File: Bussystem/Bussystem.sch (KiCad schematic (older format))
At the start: 11 parts, among them J1 PCIE-098-02-X-D-TH, J2 PCIE-098-02-X-D-TH, J3 PCIE-098-02-X-D-TH, J4 PCIE-098-02-X-D-TH, J5 PCIE-098-02-X-D-TH, J6 PCIE-098-02-X-D-EMS2-BG, J7 8x Edge conn

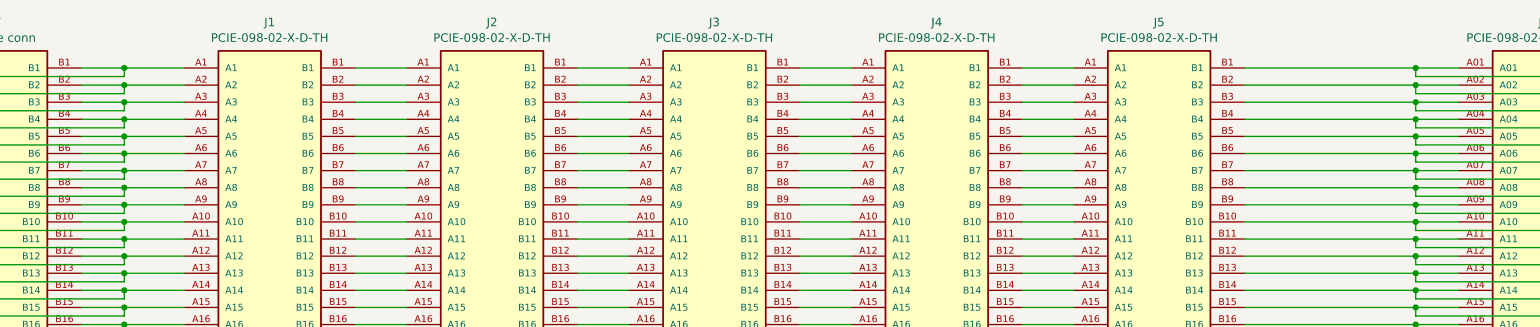
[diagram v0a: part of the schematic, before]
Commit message: lanes
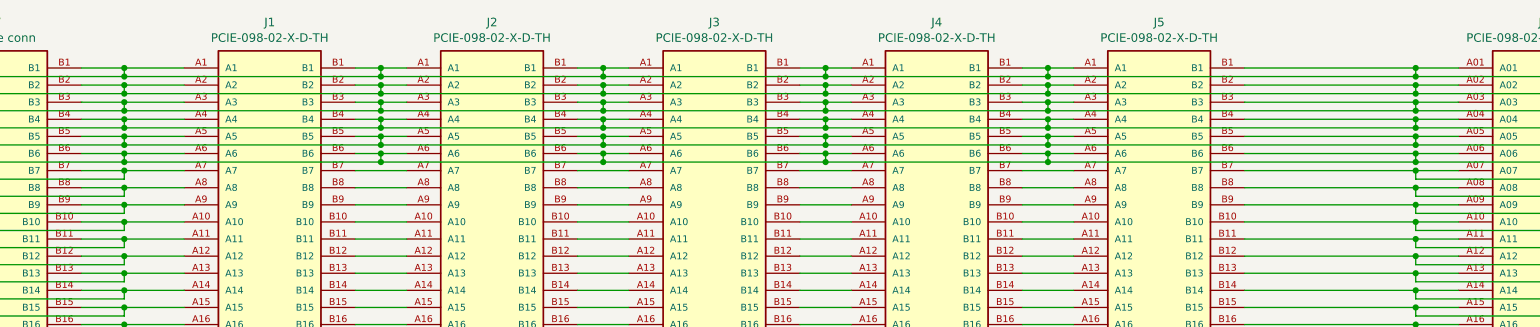
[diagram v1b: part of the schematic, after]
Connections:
- net at J1.A1, J7.A1, J7.B1: now also J1.B1, J2.A1, J2.B1, J3.A1, J3.B1, J4.A1, J4.B1, J5.A1, J5.B1, J6.A01, J6.B01
- net at J1.A2, J7.A2, J7.B2: now also J1.B2, J2.A2, J2.B2, J3.A2, J3.B2, J4.A2, J4.B2, J5.A2, J5.B2, J6.A02, J6.B02
- net at J1.A3, J7.A3, J7.B3: now also J1.B3, J2.A3, J2.B3, J3.A3, J3.B3, J4.A3, J4.B3, J5.A3, J5.B3, J6.A03, J6.B03
- net at J1.A4, J7.A4, J7.B4: now also J1.B4, J2.A4, J2.B4, J3.A4, J3.B4, J4.A4, J4.B4, J5.A4, J5.B4, J6.A04, J6.B04
- net at J1.A5, J7.A5, J7.B5: now also J1.B5, J2.A5, J2.B5, J3.A5, J3.B5, J4.A5, J4.B5, J5.A5, J5.B5, J6.A05, J6.B05
- net at J1.A6, J7.A6, J7.B6: now also J1.B6, J2.A6, J2.B6, J3.A6, J3.B6, J4.A6, J4.B6, J5.A6, J5.B6, J6.A06, J6.B06

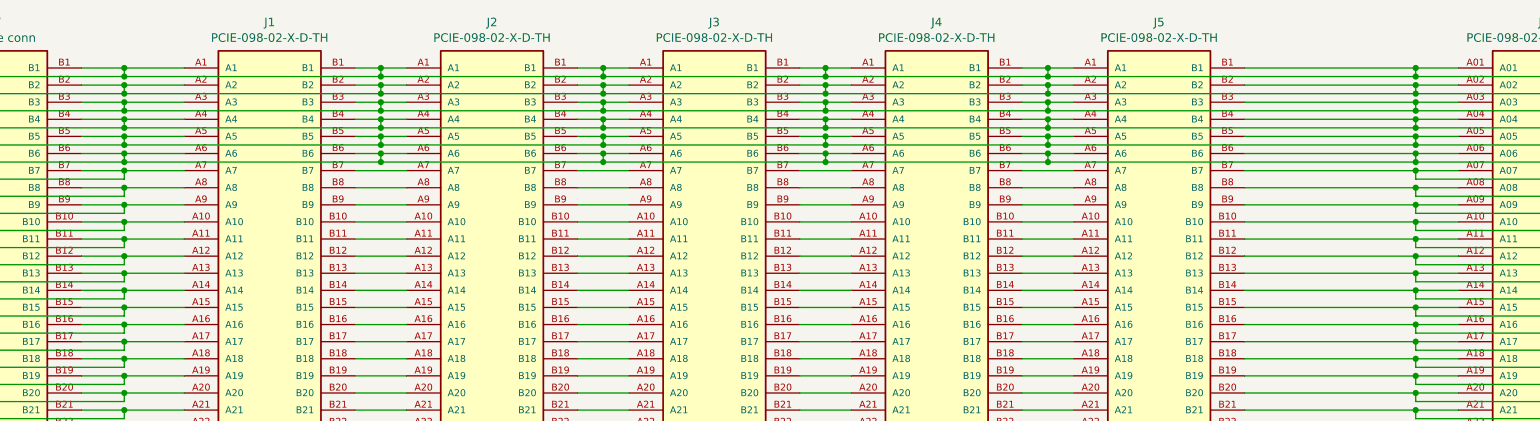
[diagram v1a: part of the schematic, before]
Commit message: some step files and additional editing of the sch
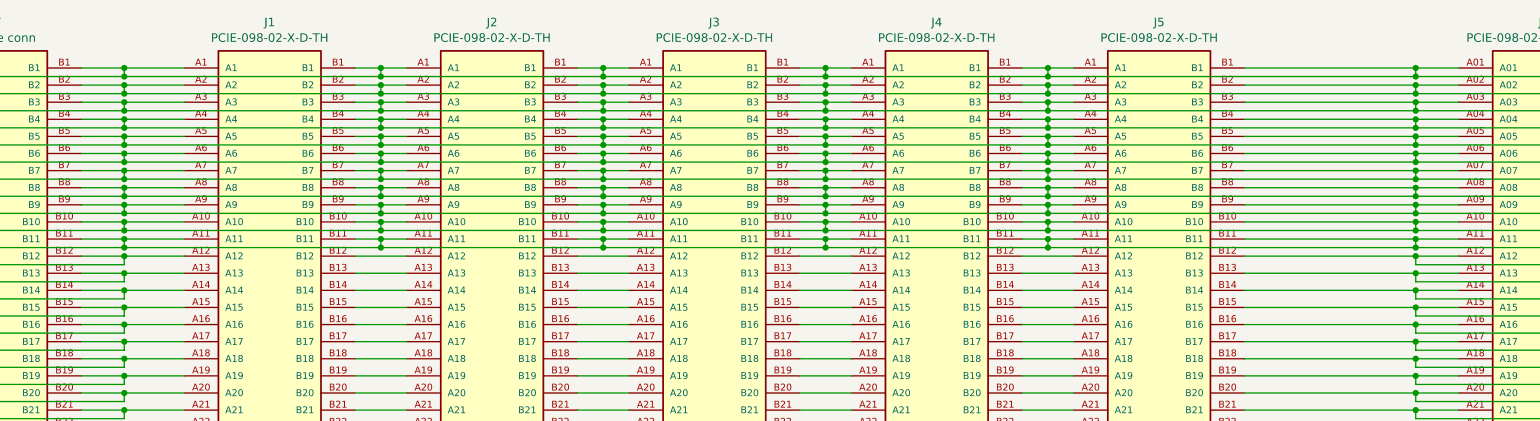
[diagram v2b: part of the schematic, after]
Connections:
- net at J1.A10, J7.A10, J7.B10: now also J1.B10, J2.A10, J2.B10, J3.A10, J3.B10, J4.A10, J4.B10, J5.A10, J5.B10, J6.A10, J6.B10
- net at J1.A11, J7.A11, J7.B11: now also J1.B11, J2.A11, J2.B11, J3.A11, J3.B11, J4.A11, J4.B11, J5.A11, J5.B11, J6.A11, J6.B11
- net at J1.A7, J7.A7, J7.B7: now also J1.B7, J2.A7, J2.B7, J3.A7, J3.B7, J4.A7, J4.B7, J5.A7, J5.B7, J6.A07, J6.B07
- net at J1.A8, J7.A8, J7.B8: now also J1.B8, J2.A8, J2.B8, J3.A8, J3.B8, J4.A8, J4.B8, J5.A8, J5.B8, J6.A08, J6.B08
- net at J1.A9, J7.A9, J7.B9: now also J1.B9, J2.A9, J2.B9, J3.A9, J3.B9, J4.A9, J4.B9, J5.A9, J5.B9, J6.A09, J6.B09
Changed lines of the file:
@@
 	3400 1550 3550 1550
 Wire Wire Line
-	3700 1650 3400 1650
-Wire Wire Line
-	3400 1750 3700 1750
-Wire Wire Line
-	3700 1850 3400 1850
-Wire Wire Line
-	3400 1950 3700 1950
-Wire Wire Line
-	3700 2050 3400 2050
+	3700 1650 3550 1650
+Wire Wire Line
+	3400 1750 3550 1750
+Wire Wire Line
+	3700 1850 3550 1850
+Wire Wire Line
+	3400 1950 3550 1950
+Wire Wire Line
+	3700 2050 3550 2050
 Wire Wire Line
 	3400 2150 3700 2150
@@
 	4700 1550 4850 1550
 Wire Wire Line
-	5000 1650 4700 1650
-Wire Wire Line
-	4700 1750 5000 1750
-Wire Wire Line
-	5000 1850 4700 1850
-Wire Wire Line
-	4700 1950 5000 1950
-Wire Wire Line
-	5000 2050 4700 2050
+	5000 1650 4850 1650
+Wire Wire Line
+	4700 1750 4850 1750
+Wire Wire Line
+	5000 1850 4850 1850
+Wire Wire Line
+	4700 1950 4850 1950
+Wire Wire Line
+	5000 2050 4850 2050
 Wire Wire Line
 	4700 2150 5000 2150
@@
 	6000 1550 6150 1550
 Wire Wire Line
-	6300 1650 6000 1650
-Wire Wire Line
-	6000 1750 6300 1750
-Wire Wire Line
-	6300 1850 6000 1850
-Wire Wire Line
-	6000 1950 6300 1950
-Wire Wire Line
-	6300 2050 6000 2050
+	6300 1650 6150 1650
+Wire Wire Line
+	6000 1750 6150 1750
+Wire Wire Line
+	6300 1850 6150 1850
+Wire Wire Line
+	6000 1950 6150 1950
+Wire Wire Line
+	6300 2050 6150 2050
 Wire Wire Line
 	6000 2150 6300 2150
@@
 	7300 1550 7450 1550
 Wire Wire Line
-	7600 1650 7300 1650
-Wire Wire Line
-	7300 1750 7600 1750
-Wire Wire Line
-	7600 1850 7300 1850
-Wire Wire Line
-	7300 1950 7600 1950
-Wire Wire Line
-	7600 2050 7300 2050
+	7600 1650 7450 1650
+Wire Wire Line
+	7300 1750 7450 1750
+Wire Wire Line
+	7600 1850 7450 1850
+Wire Wire Line
+	7300 1950 7450 1950
+Wire Wire Line
+	7600 2050 7450 2050
 Wire Wire Line
 	7300 2150 7600 2150
@@
 Wire Wire Line
 	3550 1550 3700 1550
+Wire Wire Line
+	2050 1700 3550 1700
+Connection ~ 2050 1700
+Connection ~ 9600 1700
+Wire Wire Line
+	3550 1700 3550 1650
+Connection ~ 3550 1700
+Wire Wire Line
+	3550 1700 4850 1700
+Connection ~ 3550 1650
+Wire Wire Line
+	3550 1650 3400 1650
+Wire Wire Line
+	4850 1700 4850 1650
+Connection ~ 4850 1700
+Wire Wire Line
+	4850 1700 6150 1700
+Connection ~ 4850 1650
+Wire Wire Line
+	4850 1650 4700 1650
+Wire Wire Line
+	6150 1700 6150 1650
+Connection ~ 6150 1700
+Wire Wire Line
+	6150 1700 7450 1700
+Connection ~ 6150 1650
+Wire Wire Line
+	6150 1650 6000 1650
+Wire Wire Line
+	7450 1700 7450 1650
+Connection ~ 7450 1700
+Wire Wire Line
+	7450 1700 9600 1700
+Connection ~ 7450 1650
+Wire Wire Line
+	7450 1650 7300 1650
+Wire Wire Line
+	2050 1800 3550 1800
+Wire Wire Line
+	3550 1800 3550 1750
+Connection ~ 2050 1800
+Connection ~ 3550 1750
+Wire Wire Line
+	3550 1750 3700 1750
+Wire Wire Line
+	3550 1800 4850 1800
+Wire Wire Line
+	4850 1800 4850 1750
+Connection ~ 3550 1800
+Connection ~ 4850 1750
+Wire Wire Line
+	4850 1750 5000 1750
+Wire Wire Line
+	4850 1800 6150 1800
+Wire Wire Line
+	6150 1800 6150 1750
+Connection ~ 4850 1800
+Connection ~ 6150 1750
+Wire Wire Line
+	6150 1750 6300 1750
+Wire Wire Line
+	6150 1800 7450 1800
+Wire Wire Line
+	7450 1800 7450 1750
+Connection ~ 6150 1800
+Connection ~ 7450 1750
+Wire Wire Line
+	7450 1750 7600 1750
+Wire Wire Line
+	7450 1800 9600 1800
+Connection ~ 7450 1800
+Connection ~ 9600 1800
+Wire Wire Line
+	2050 1900 3550 1900
+Connection ~ 2050 1900
+Connection ~ 9600 1900
+Wire Wire Line
+	7450 1900 7450 1850
+Connection ~ 7450 1900
+Wire Wire Line
+	7450 1900 9600 1900
+Connection ~ 7450 1850
+Wire Wire Line
+	7450 1850 7300 1850
+Wire Wire Line
+	6150 1900 6150 1850
+Connection ~ 6150 1900
+Wire Wire Line
+	6150 1900 7450 1900
+Connection ~ 6150 1850
+Wire Wire Line
+	6150 1850 6000 1850
+Wire Wire Line
+	3550 1900 3550 1850
+Connection ~ 3550 1900
+Wire Wire Line
+	3550 1900 4850 1900
+Connection ~ 3550 1850
+Wire Wire Line
+	3550 1850 3400 1850
+Wire Wire Line
+	4850 1900 4850 1850
+Connection ~ 4850 1900
+Wire Wire Line
+	4850 1900 6150 1900
+Connection ~ 4850 1850
+Wire Wire Line
+	4850 1850 4700 1850
+Wire Wire Line
+	2050 2000 3550 2000
+Wire Wire Line
+	3550 2000 3550 1950
+Connection ~ 2050 2000
+Connection ~ 3550 1950
+Wire Wire Line
+	3550 1950 3700 1950
+Wire Wire Line
+	3550 2000 4850 2000
+Connection ~ 3550 2000
+Connection ~ 9600 2000
+Wire Wire Line
+	7450 2000 7450 1950
+Connection ~ 7450 2000
+Wire Wire Line
+	7450 2000 9600 2000
+Connection ~ 7450 1950
+Wire Wire Line
+	7450 1950 7600 1950
+Wire Wire Line
+	6150 2000 6150 1950
+Connection ~ 6150 2000
+Wire Wire Line
+	6150 2000 7450 2000
+Connection ~ 6150 1950
+Wire Wire Line
+	6150 1950 6300 1950
+Wire Wire Line
+	4850 2000 4850 1950
+Connection ~ 4850 2000
+Wire Wire Line
+	4850 2000 6150 2000
+Connection ~ 4850 1950
+Wire Wire Line
+	4850 1950 5000 1950
+Wire Wire Line
+	2050 2100 3550 2100
+Connection ~ 2050 2100
+Connection ~ 9600 2100
+Wire Wire Line
+	7450 2100 7450 2050
+Connection ~ 7450 2100
+Wire Wire Line
+	7450 2100 9600 2100
+Connection ~ 7450 2050
+Wire Wire Line
+	7450 2050 7300 2050
+Wire Wire Line
+	6150 2100 6150 2050
+Connection ~ 6150 2100
+Wire Wire Line
+	6150 2100 7450 2100
+Connection ~ 6150 2050
+Wire Wire Line
+	6150 2050 6000 2050
+Wire Wire Line
+	3550 2100 3550 2050
+Connection ~ 3550 2100
+Wire Wire Line
+	3550 2100 4850 2100
+Connection ~ 3550 2050
+Wire Wire Line
+	3550 2050 3400 2050
+Wire Wire Line
+	4850 2100 4850 2050
+Connection ~ 4850 2100
+Wire Wire Line
+	4850 2100 6150 2100
+Connection ~ 4850 2050
+Wire Wire Line
+	4850 2050 4700 2050
 $EndSCHEMATC
